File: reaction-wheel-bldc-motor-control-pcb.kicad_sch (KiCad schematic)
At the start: 34 parts, among them J1 USB_C_Receptacle_USB2.0_16P, J7 Conn_01x04_Pin, J8 Conn_01x04_Pin, SW1 SW_SPDT, SW3 SW_SPST, U1 STM32G431CBUx, U2 AS5047D, U3 DRV8311H, U5 USBLC6-2SC6, U7 TJA1051T-3, Y1 16MHz

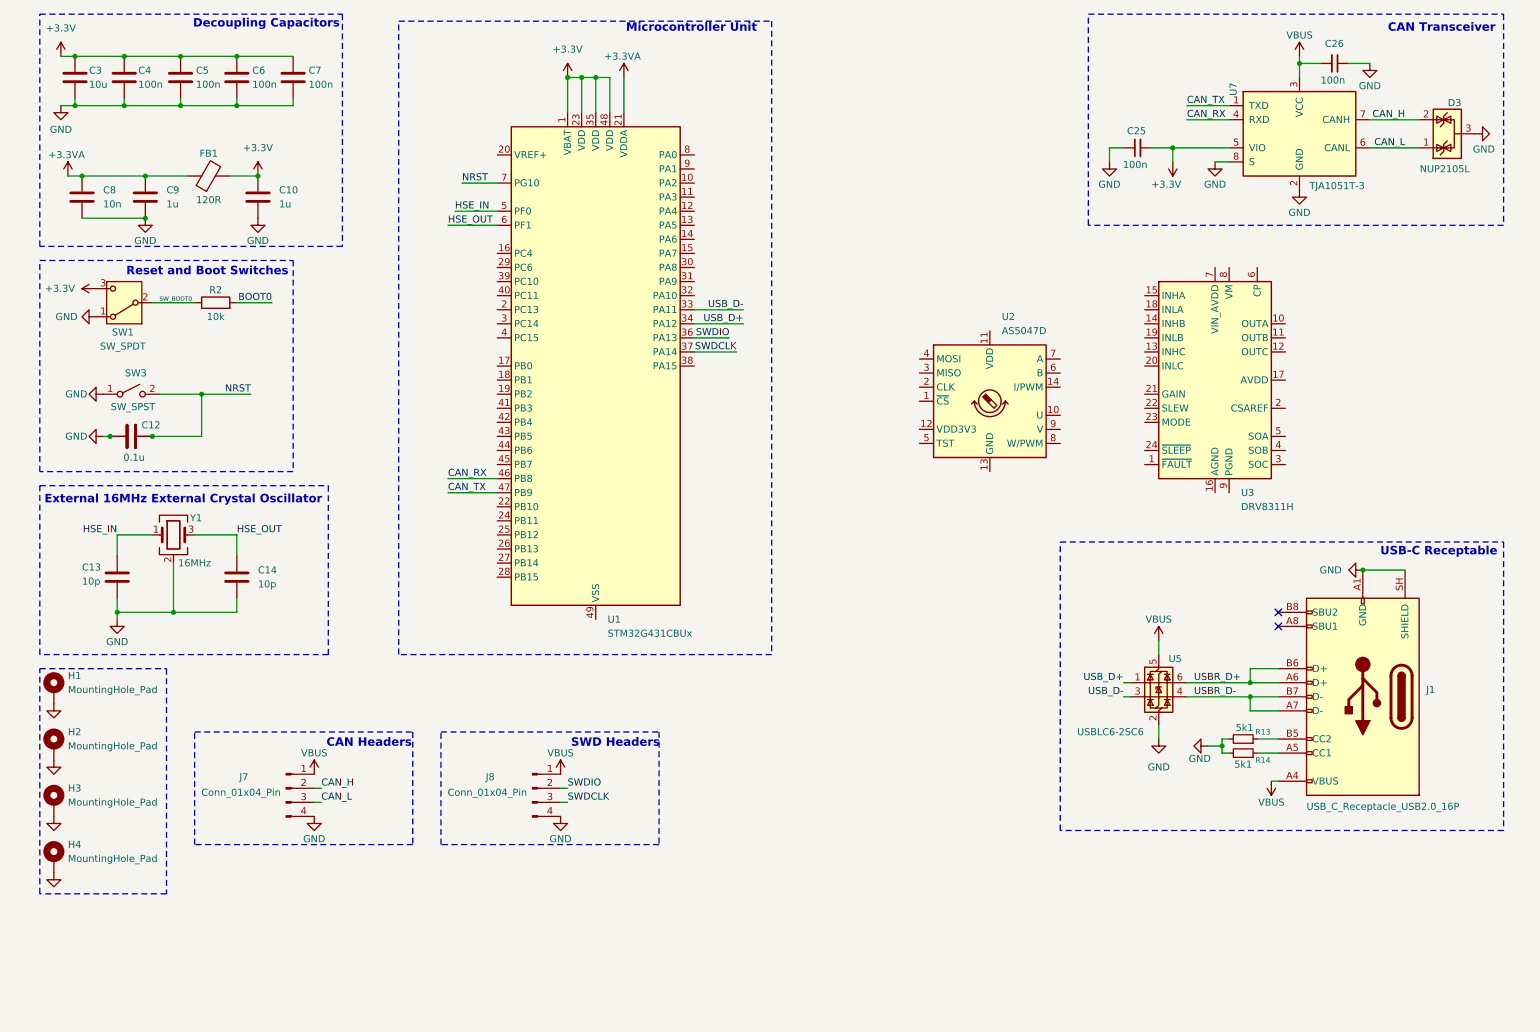
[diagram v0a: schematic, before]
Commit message: schematic almost complete
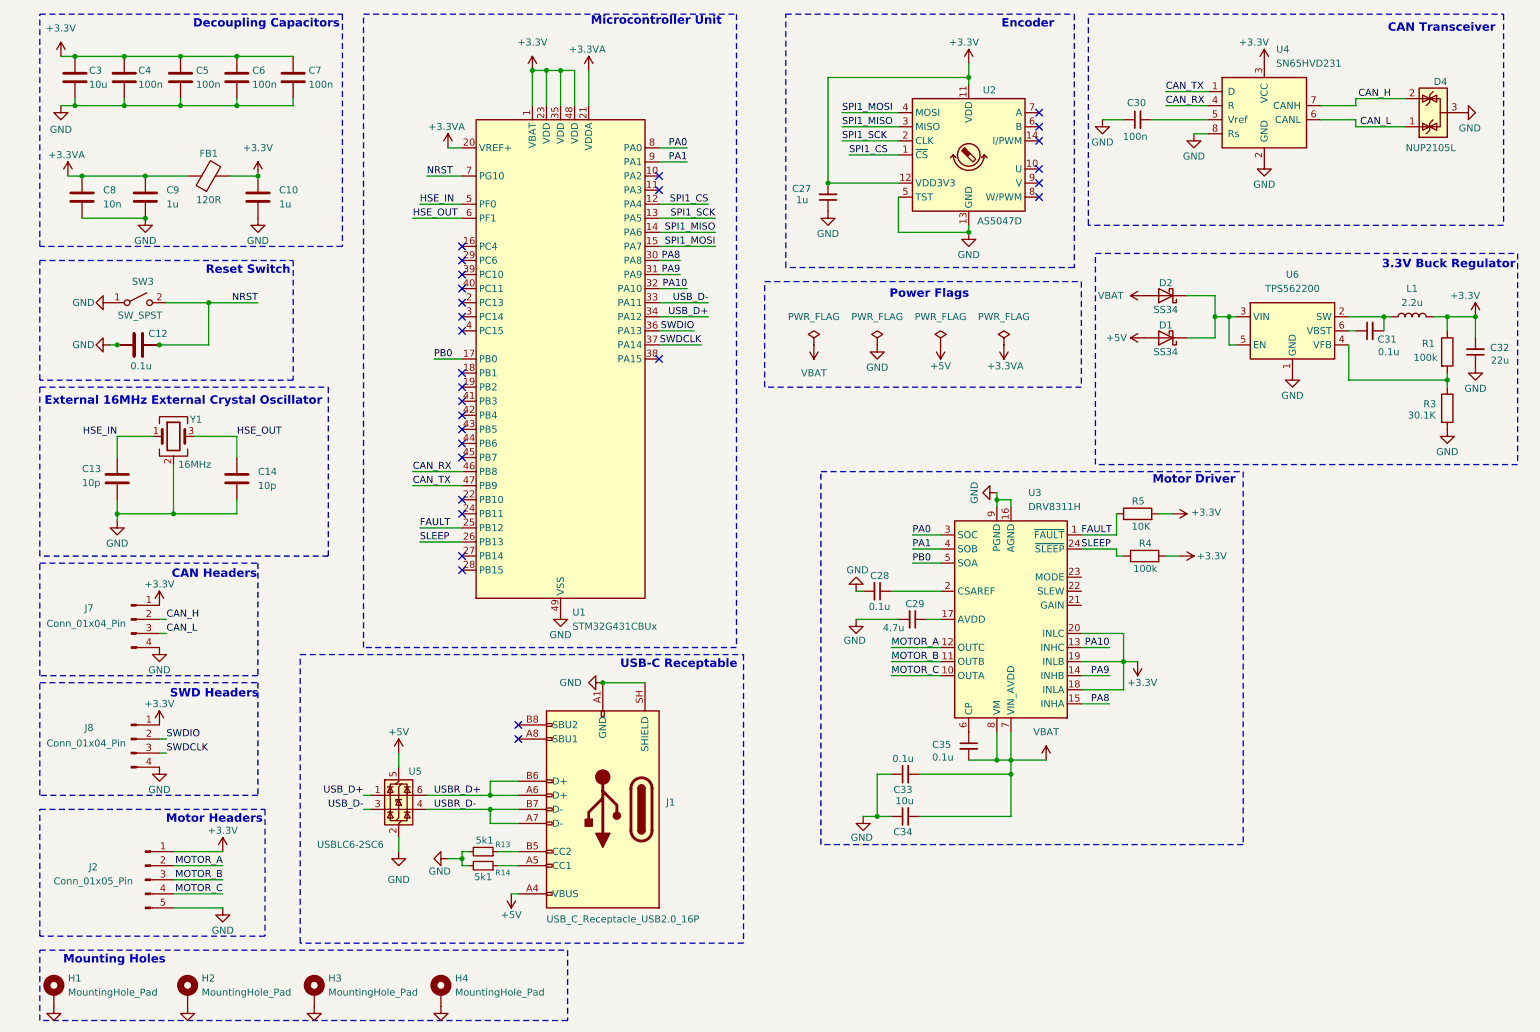
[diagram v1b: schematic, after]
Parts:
- removed C25, C26: 100n, Capacitor_SMD:C_0805_2012Metric_Pad1.18x1.45mm_HandSolder, symbol Device:C_Small
- removed D3: NUP2105L, Package_TO_SOT_SMD:SOT-23, symbol Power_Protection:NUP2105L
- removed R2: 10k, Resistor_SMD:R_0402_1005Metric, symbol Device:R
- removed SW1: SW_SPDT, Button_Switch_THT:SW_E-Switch_EG1224_SPDT_Angled, symbol Switch:SW_SPDT
- removed U7: TJA1051T-3, Package_SO:SOIC-8_3.9x4.9mm_P1.27mm, symbol Interface_CAN_LIN:TJA1051T-3
- added C27: 1u, Capacitor_SMD:C_0805_2012Metric_Pad1.18x1.45mm_HandSolder, symbol Device:C_Small
- added C28, C31, C33, C35: 0.1u, Capacitor_SMD:C_0805_2012Metric_Pad1.18x1.45mm_HandSolder, symbol Device:C_Small
- added C29: 4.7u, Capacitor_SMD:C_0805_2012Metric_Pad1.18x1.45mm_HandSolder, symbol Device:C_Small
- added C30: 100n, Capacitor_SMD:C_0805_2012Metric_Pad1.18x1.45mm_HandSolder, symbol Device:C_Small
- added C32: 22u, Capacitor_SMD:C_0805_2012Metric_Pad1.18x1.45mm_HandSolder, symbol Device:C_Small
- added C34: 10u, Capacitor_SMD:C_0805_2012Metric_Pad1.18x1.45mm_HandSolder, symbol Device:C_Small
- added D1, D2: SS34, Diode_SMD:D_SMA, symbol Diode:SS34
- added D4: NUP2105L, Package_TO_SOT_SMD:SOT-23, symbol Power_Protection:NUP2105L
- added J2: Conn_01x05_Pin, symbol Connector:Conn_01x05_Pin
- added L1: 2.2u, symbol Device:L
- added R1, R4: 100k, symbol Device:R
- added R3: 30.1K, symbol Device:R
- added R5: 10K, symbol Device:R
- added U4: SN65HVD231, Package_SO:SOIC-8_3.9x4.9mm_P1.27mm, symbol Interface_CAN_LIN:SN65HVD231
- added U6: TPS562200, Package_TO_SOT_SMD:SOT-23-6, symbol Regulator_Switching:TPS562200
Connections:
- net +3.3V: now also J7.1 (Pin_1), J8.1 (Pin_1), U2.11 (VDD), U2.12 (VDD3V3), U3.18 (INLA), U3.19 (INLB), U3.20 (INLC), C27.2, C32.2, J2.1 (Pin_1), L1.2, R1.1, R4.2, R5.2, U4.3 (VCC)
- net +3.3VA: now also U1.20 (VREF+)
- net CAN_H: now also D4.2 (K), U4.7 (CANH)
- net CAN_L: now also D4.1 (K), U4.6 (CANL)
- net CAN_RX: now also U4.4 (R)
- net CAN_TX: now also U4.1 (D)
- net GND: now also U1.49 (VSS), U2.13 (GND), U2.5 (TST), U3.16 (AGND), U3.25 (PGND), U3.9 (PGND), C27.1, C28.2, C29.2, C30.1, C32.1, C33.1, C34.1, D4.3 (A), J2.5 (Pin_5), R3.2, U4.2 (GND), U4.8 (Rs), U6.1 (GND)
- net SPI1_CS: now reaches U2.1 (~{CS})
- net SPI1_CS: now also U1.12 (PA4)
- net SPI1_SCK: now reaches U2.2 (CLK)
- net SPI1_SCK: now also U1.13 (PA5)
- net SPI1_MISO: now reaches U2.3 (MISO)
- net SPI1_MISO: now also U1.14 (PA6)
- net SPI1_MOSI: now reaches U2.4 (MOSI)
- net SPI1_MOSI: now also U1.15 (PA7)
- net FAULT: now reaches U3.1 (~{FAULT})
- net FAULT: now also U1.25 (PB12), R5.1
- net MOTOR_C: now reaches U3.10 (OUTA)
- net MOTOR_C: now also J2.4 (Pin_4)
- net MOTOR_B: now reaches U3.11 (OUTB)
- net MOTOR_B: now also J2.3 (Pin_3)
- net MOTOR_A: now reaches U3.12 (OUTC)
- net MOTOR_A: now also J2.2 (Pin_2)
- net PA10: now reaches U3.13 (INHC)
- net PA10: now also U1.32 (PA10)
- net PA9: now reaches U3.14 (INHB)
- net PA9: now also U1.31 (PA9)
- net PA8: now reaches U3.15 (INHA)
- net PA8: now also U1.30 (PA8)
- net at U3.17 (AVDD): now also C29.1
- net at U3.2 (CSAREF): now also C28.1
- net SLEEP: now reaches U3.24 (~{SLEEP})
- net SLEEP: now also U1.26 (PB13), R4.1
- net PA0: now reaches U3.3 (SOC)
- net PA0: now also U1.8 (PA0)
- net PA1: now reaches U3.4 (SOB)
- net PA1: now also U1.9 (PA1)
- net PB0: now reaches U3.5 (SOA)
- net PB0: now also U1.17 (PB0)
- net at U3.6 (CP): now also C35.1
- net VBAT: now reaches U3.7 (VIN_AVDD)
- net VBAT: now also U3.8 (VM), C33.2, C34.2, C35.2, D2.2 (A)
- net VBUS renamed +5V
- net +5V: now also D1.2 (A); no longer J7.1 (Pin_1), J8.1 (Pin_1)
- new net: D1.1 (K), D2.1 (K), U6.3 (VIN), U6.5 (EN)
- new net: R1.2, R3.1, U6.4 (VFB)
- new net: C31.2, L1.1, U6.2 (SW)
- new net: C31.1, U6.6 (VBST)
- new net: C30.2, U4.5 (Vref)
- no-connect marks 2 -> 29
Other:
- note added: "3.3V Buck Regulator"
- note added: "Encoder"
- note added: "Motor Driver"
- note added: "Motor Headers"
- note added: "Mounting Holes"
- note added: "Power Flags"
- note added: "Reset Switch"
- note removed: "Reset and Boot Switches"
- moved on the sheet: C12, C13, C14, H1, H2, H3, H4, J1, J7, J8, R13, R14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
